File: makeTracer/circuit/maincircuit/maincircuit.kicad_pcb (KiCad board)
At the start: 2 copper layers, 20.3 x 8.4 mm, 33 parts, among them IC1 PIC16F1778-I/SP, J1 PICKit3, J2 Sensor, J3 I^{2}C, J4 LED, J5 Motor_L, J6 Motor_R, J7 Bus_PCI_Express_x1_Debug, Q1 MP4212, Q2 MP4212, SW1 SW_DPDT_x2, SW2 Reset, SW3 Red, SW4 Green, U1 74HC00

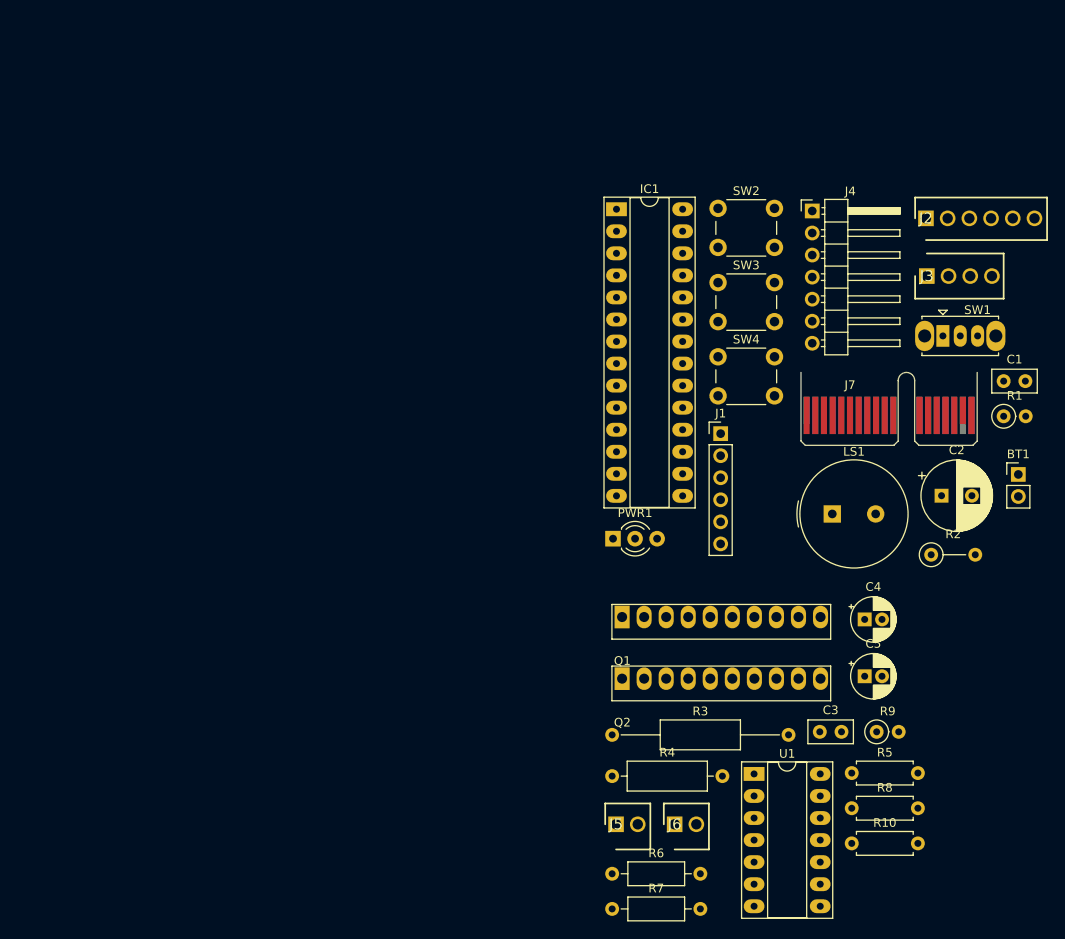
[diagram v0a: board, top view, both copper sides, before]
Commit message: complete: circuit
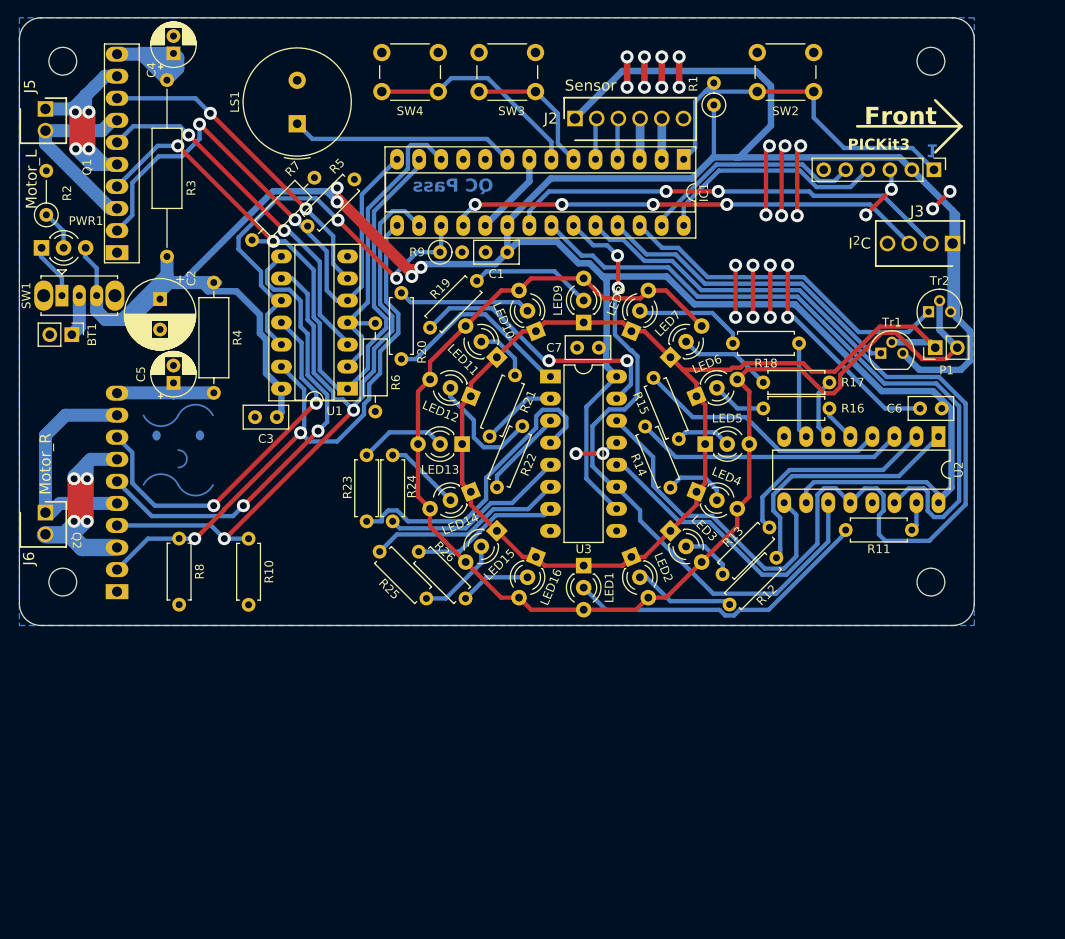
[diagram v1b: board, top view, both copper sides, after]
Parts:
- removed J4: LED, Connector_PinHeader_2.54mm:PinHeader_1x07_P2.54mm_Horizontal
- removed J7: Bus_PCI_Express_x1_Debug, Connector_PCBEdge:BUS_PCIexpress_x1
- added C6: 0.1u_pass, Capacitor_THT:C_Disc_D5.0mm_W2.5mm_P2.50mm, F.Cu at (126.2, 64.9)
- added C7: 0.1u_pass, Capacitor_THT:C_Disc_D5.0mm_W2.5mm_P2.50mm, F.Cu at (86.8, 57.9)
- added LED1: Circle, LED_THT:LED_D3.0mm-3, F.Cu at (85.0, 83.0)
- added LED10: Circle, LED_THT:LED_D3.0mm-3, F.Cu at (79.5, 56.0)
- added LED11: Circle, LED_THT:LED_D3.0mm-3, F.Cu at (75.0, 59.0)
- added LED12: Circle, LED_THT:LED_D3.0mm-3, F.Cu at (72.0, 63.5)
- added LED13: Circle, LED_THT:LED_D3.0mm-3, F.Cu at (71.0, 69.0)
- added LED14: Circle, LED_THT:LED_D3.0mm-3, F.Cu at (72.0, 74.5)
- added LED15: Circle, LED_THT:LED_D3.0mm-3, F.Cu at (75.0, 79.0)
- added LED16: Circle, LED_THT:LED_D3.0mm-3, F.Cu at (79.5, 82.0)
- added LED2: Circle, LED_THT:LED_D3.0mm-3, F.Cu at (90.5, 82.0)
- added LED3: Circle, LED_THT:LED_D3.0mm-3, F.Cu at (95.0, 79.0)
- added LED4: Circle, LED_THT:LED_D3.0mm-3, F.Cu at (98.0, 74.5)
- added LED5: Circle, LED_THT:LED_D3.0mm-3, F.Cu at (99.0, 69.0)
- added LED6: Circle, LED_THT:LED_D3.0mm-3, F.Cu at (98.0, 63.5)
- added LED7: Circle, LED_THT:LED_D3.0mm-3, F.Cu at (95.0, 59.0)
- added LED8: Circle, LED_THT:LED_D3.0mm-3, F.Cu at (90.5, 56.0)
- added LED9: Circle, LED_THT:LED_D3.0mm-3, F.Cu at (85.0, 55.0)
- added P1: FrontsidePort, Connector_PinHeader_2.54mm:PinHeader_1x02_P2.54mm_Vertical, F.Cu at (125.5, 57.9)
- added R11: 470, Resistor_THT:R_Axial_DIN0207_L6.3mm_D2.5mm_P7.62mm_Horizontal, F.Cu at (115.2, 78.9)
- added R12: 470, Resistor_THT:R_Axial_DIN0207_L6.3mm_D2.5mm_P7.62mm_Horizontal, F.Cu at (101.8, 87.5)
- added R13: 470, Resistor_THT:R_Axial_DIN0207_L6.3mm_D2.5mm_P7.62mm_Horizontal, F.Cu at (101.0, 84.0)
- added R14: 470, Resistor_THT:R_Axial_DIN0207_L6.3mm_D2.5mm_P7.62mm_Horizontal, F.Cu at (95.0, 74.0)
- added R15: 470, Resistor_THT:R_Axial_DIN0207_L6.3mm_D2.5mm_P7.62mm_Horizontal, F.Cu at (96.0, 68.4)
- added R16: 470, Resistor_THT:R_Axial_DIN0207_L6.3mm_D2.5mm_P7.62mm_Horizontal, F.Cu at (105.7, 64.9)
- added R17: 470, Resistor_THT:R_Axial_DIN0207_L6.3mm_D2.5mm_P7.62mm_Horizontal, F.Cu at (105.7, 61.9)
- added R18: 470, Resistor_THT:R_Axial_DIN0207_L6.3mm_D2.5mm_P7.62mm_Horizontal, F.Cu at (102.2, 57.4)
- added R19: 470, Resistor_THT:R_Axial_DIN0207_L6.3mm_D2.5mm_P7.62mm_Horizontal, F.Cu at (72.7, 50.2)
- added R20: 470, Resistor_THT:R_Axial_DIN0207_L6.3mm_D2.5mm_P7.62mm_Horizontal, F.Cu at (64.0, 51.6)
- added R21: 470, Resistor_THT:R_Axial_DIN0207_L6.3mm_D2.5mm_P7.62mm_Horizontal, F.Cu at (77.1, 61.1)
- added R22: 470, Resistor_THT:R_Axial_DIN0207_L6.3mm_D2.5mm_P7.62mm_Horizontal, F.Cu at (77.9, 66.9)
- added R23: 470, Resistor_THT:R_Axial_DIN0207_L6.3mm_D2.5mm_P7.62mm_Horizontal, F.Cu at (60.0, 70.3)
- added R24: 470, Resistor_THT:R_Axial_DIN0207_L6.3mm_D2.5mm_P7.62mm_Horizontal, F.Cu at (63.0, 70.3)
- added R25: 470, Resistor_THT:R_Axial_DIN0207_L6.3mm_D2.5mm_P7.62mm_Horizontal, F.Cu at (66.9, 86.8)
- added R26: 470, Resistor_THT:R_Axial_DIN0207_L6.3mm_D2.5mm_P7.62mm_Horizontal, F.Cu at (71.4, 86.8)
- added REF**: MountingHole_3.2mm_M3, MountingHole:MountingHole_3.2mm_M3, F.Cu at (125.0, 24.9)
- added REF**: MountingHole_3.2mm_M3, MountingHole:MountingHole_3.2mm_M3, F.Cu at (25.0, 84.9)
- added REF**: MountingHole_3.2mm_M3, MountingHole:MountingHole_3.2mm_M3, F.Cu at (25.0, 24.9)
- added REF**: MountingHole_3.2mm_M3, MountingHole:MountingHole_3.2mm_M3, F.Cu at (125.0, 84.9)
- added REF**: KiCad-Logo2_8mm_SilkScreen, Symbol:KiCad-Logo2_8mm_SilkScreen, B.Cu at (52.0, 78.9)
- added Tr1: DTC114E, Package_TO_SOT_THT:TO-92, F.Cu at (119.2, 58.5)
- added Tr2: DTC114E, Package_TO_SOT_THT:TO-92, F.Cu at (124.7, 53.8)
- added U2: 74HC595, Package_DIP:DIP-16_W7.62mm_LongPads, F.Cu at (125.9, 68.1)
- added U3: 74HC595, Package_DIP:DIP-16_W7.62mm_LongPads, F.Cu at (81.2, 61.2)
- Q2: moved to B.Cu
- moved BT1 110.2 mm to (26.0, 56.4), turned to -90 degrees
- moved R2 109.2 mm to (23.1, 42.6), turned to 90 degrees
- moved J5 105.4 mm to (23.0, 30.4), turned to -90 degrees
- moved C4 102.9 mm to (37.8, 24.0), turned to 90 degrees
- moved SW1 101.6 mm to (24.9, 51.9)
- moved C2 92.8 mm to (36.2, 52.3), turned to -90 degrees
- moved R5 88.9 mm to (53.2, 43.9), turned to 45 degrees
- moved R7 87.5 mm to (46.8, 45.5), turned to 45 degrees
- moved C5 86.5 mm to (37.8, 62.0), turned to 90 degrees
- moved R8 83.5 mm to (38.4, 79.9), turned to -90 degrees
- moved J6 80.9 mm to (23.0, 76.9), turned to -90 degrees
- moved R10 77.8 mm to (46.4, 79.9), turned to -90 degrees
- moved LS1 76.3 mm to (52.0, 32.1), turned to 90 degrees
- moved R3 75.3 mm to (37.0, 47.4), turned to 90 degrees
- moved R9 74.7 mm to (68.5, 46.9)
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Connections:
- IC1 pad 22: LED_Data -> /16x2LEDs/Data
- IC1 pad 23: LED_Clock -> /16x2LEDs/Clock
- IC1 pad 24: LED_Flash -> /16x2LEDs/Flash
- IC1 pad 25: LED_ColorR -> /16x2LEDs/Select_Red
- IC1 pad 26: LED_ColorG -> /16x2LEDs/Select_Green
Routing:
- net VDD: track 0.00 -> 387.2 mm, vias 0 -> 4
- net /16x2LEDs/Green_Src: track 0.00 -> 158.6 mm
- net /16x2LEDs/Red_Src: track 0.00 -> 131.4 mm
- net /16x2LEDs/Flash: track 0.00 -> 124.7 mm
- net GND: track 0.00 -> 106.5 mm, vias 0 -> 28
- net /Motordrive/R_SEL1: track 0.00 -> 86.7 mm, vias 0 -> 2
- net /Motordrive/L_SEL1: track 0.00 -> 80.3 mm, vias 0 -> 2
- net /16x2LEDs/Data: track 0.00 -> 78.0 mm
- net /16x2LEDs/Clock: track 0.00 -> 77.1 mm, vias 0 -> 2
- net /Motordrive/R_SEL2: track 0.00 -> 71.7 mm, vias 0 -> 2
- net /Motordrive/L_SEL2: track 0.00 -> 64.7 mm, vias 0 -> 2
- net I^{2}C_SCL: track 0.00 -> 54.9 mm, vias 0 -> 4
- net Net-(Q2-G_3): track 0.00 -> 54.0 mm, vias 0 -> 2
- net I^{2}C_SDA: track 0.00 -> 52.2 mm, vias 0 -> 2
- net /Motordrive/R_PWM: track 0.00 -> 49.8 mm, vias 0 -> 2
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- added copper zone on B.Cu, net GND
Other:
- board size 20.3 x 8.4 mm -> 110 x 70 mm
- board text added: "1"
- board text added: "Front"
- board text added: "PICKit3 Size"
- board text added: "QC Pass"
